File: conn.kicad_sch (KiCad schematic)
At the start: 57 parts, among them J1 JST_1x02, J10 MicroFit_2x04, J11 MLX_1x03, J12 MLX_1x03, J13 JST_1x04, J14 JST_1x04, J15 JST_1x04, J16 JST_1x04, J17 JST_1x02, J5 JST_01x02, J7 JST_B6B-XH, J8 MicroFit_2x04, J9 MicroFit_2x04, SW2 !EMERG STOP!

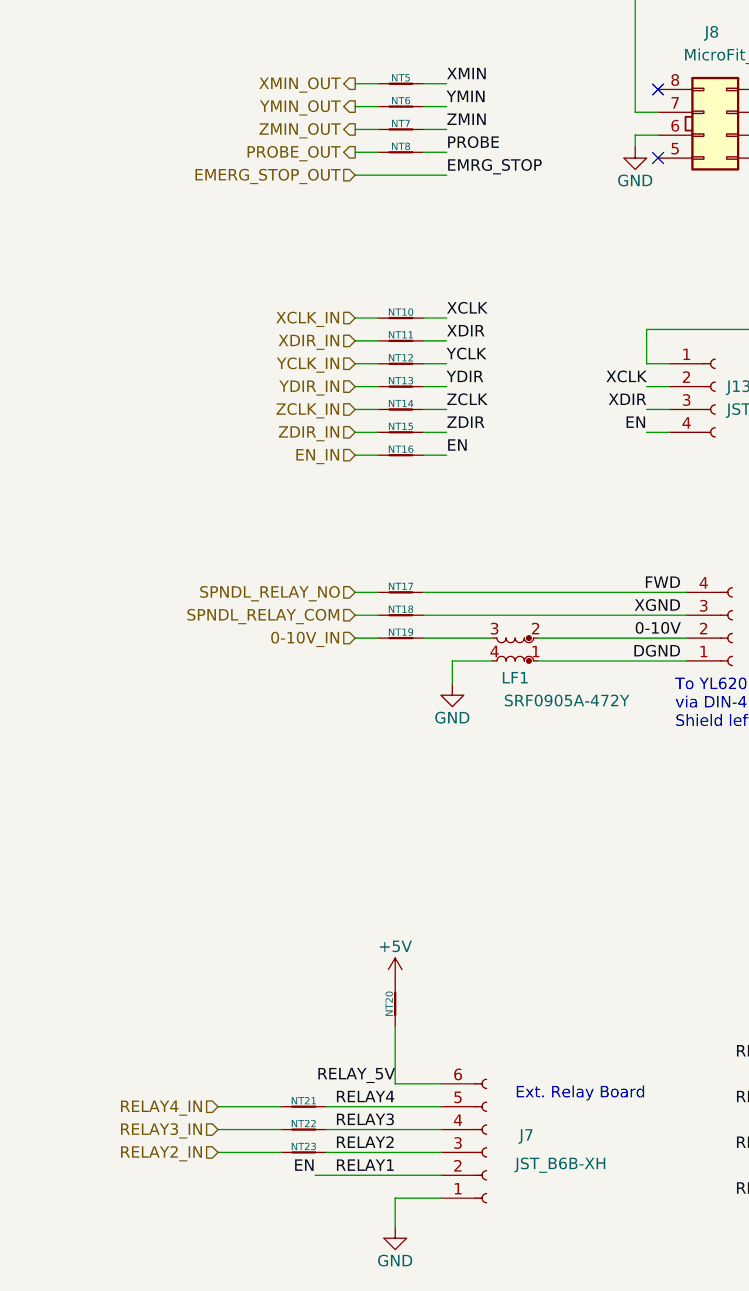
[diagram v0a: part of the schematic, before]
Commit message: Forgot R1 and more NT fun.
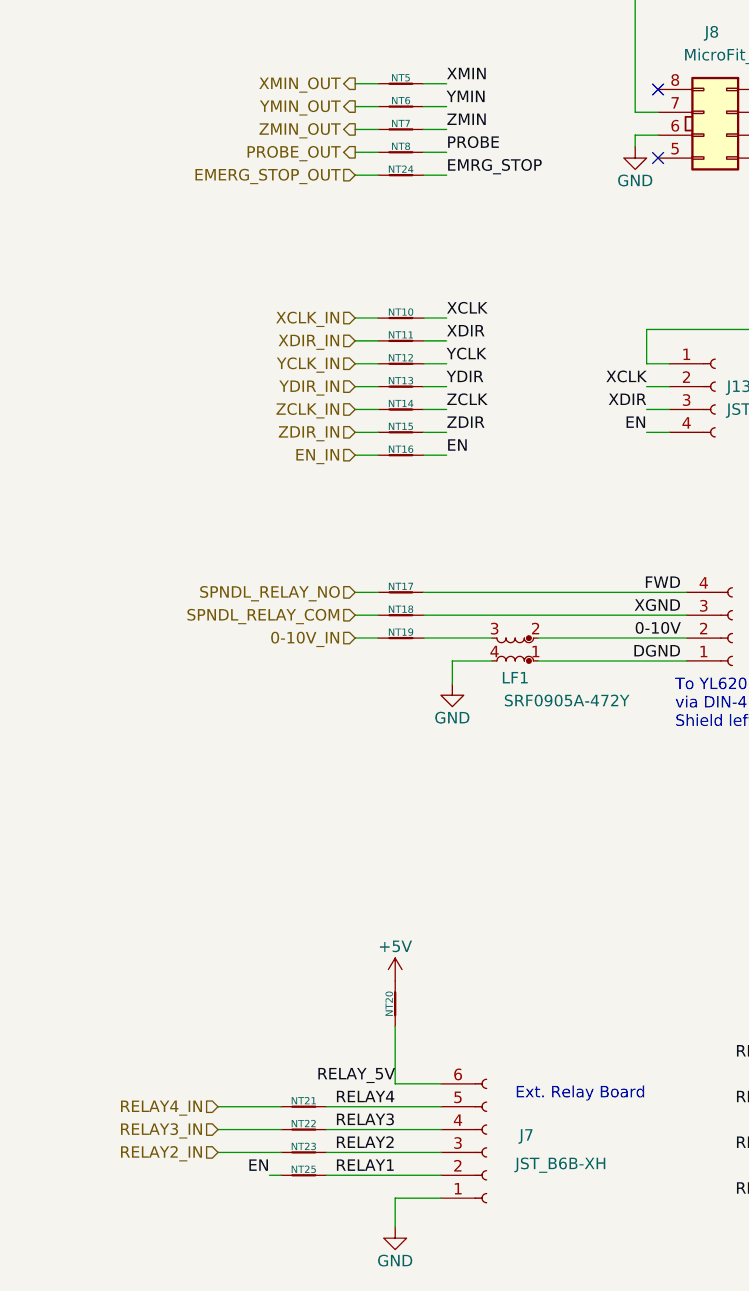
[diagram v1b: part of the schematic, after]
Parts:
- added NT24, NT25: DNI, _footprints:NetTie-2_SMD_Pad0.3mm, symbol Device:NetTie_2
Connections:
- net EMERG_STOP_OUT: now also NT24.1; no longer J1.2 (Pin_2)
- net EN: now also NT25.1; no longer D20.1 (K), J7.2 (Pin_2)
- new net EMRG_STOP: J1.2 (Pin_2), NT24.2
- new net RELAY1: D20.1 (K), J7.2 (Pin_2), NT25.2
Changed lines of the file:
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@@
+    (stroke (width 0) (type default) (color 0 0 0 0))
+  )
+  (wire (pts (xy 53.34 172.72) (xy 66.04 172.72))
     (stroke (width 0) (type default) (color 0 0 0 0))
   )
@@
     (stroke (width 0) (type default) (color 0 0 0 0))
   )
-  (wire (pts (xy 56.515 61.595) (xy 66.675 61.595))
+  (wire (pts (xy 56.515 61.595) (xy 59.055 61.595))
     (stroke (width 0) (type default) (color 0 0 0 0))
   )
@@
     (stroke (width 0) (type default) (color 0 0 0 0))
   )
+  (wire (pts (xy 46.99 172.72) (xy 48.26 172.72))
+    (stroke (width 0) (type default) (color 0 0 0 0))
+  )
   (wire (pts (xy 53.34 170.18) (xy 66.04 170.18))
     (stroke (width 0) (type default) (color 0 0 0 0))
@@
     (stroke (width 0) (type default) (color 0 0 0 0))
   )
+  (wire (pts (xy 64.135 61.595) (xy 66.675 61.595))
+    (stroke (width 0) (type default) (color 0 0 0 0))
+  )
   (wire (pts (xy 197.485 125.73) (xy 204.47 125.73))
     (stroke (width 0) (type default) (color 0 0 0 0))
@@
   )
   (wire (pts (xy 248.92 44.45) (xy 250.19 44.45))
-    (stroke (width 0) (type default) (color 0 0 0 0))
-  )
-  (wire (pts (xy 52.07 172.72) (xy 66.04 172.72))
     (stroke (width 0) (type default) (color 0 0 0 0))
   )
@@
     (effects (font (size 1.27 1.27)) (justify right bottom))
   )
-  (label "EN" (at 52.07 172.72 180)
+  (label "EN" (at 46.99 172.72 180)
     (effects (font (size 1.27 1.27)) (justify right bottom))
   )
@@
     )
     (property "Datasheet" "~" (id 3) (at 146.05 100.33 0)
+      (effects (font (size 1.27 1.27)) hide)
+    )
+    (pin "1")
+    (pin "2")
+  )
+  (symbol (lib_id "Device:NetTie_2") (at 50.8 172.72 0) (unit 1)
+    (in_bom yes) (on_board yes)
+    (property "Reference" "NT25" (id 0) (at 50.8 172.085 0)
+      (effects (font (size 0.8 0.8)))
+    )
+    (property "Value" "DNI" (id 1) (at 50.8 170.18 0)
+      (effects (font (size 1.27 1.27)) hide)
+    )
+    (property "Footprint" "_footprints:NetTie-2_SMD_Pad0.3mm" (id 2) (at 50.8 172.72 0)
+      (effects (font (size 1.27 1.27)) hide)
+    )
+    (property "Datasheet" "~" (id 3) (at 50.8 172.72 0)
       (effects (font (size 1.27 1.27)) hide)
     )
@@
       (effects (font (size 1.27 1.27)) hide)
     )
+    (pin "1")
+    (pin "2")
+  )
+  (symbol (lib_id "Device:NetTie_2") (at 61.595 61.595 0) (unit 1)
+    (in_bom yes) (on_board yes)
+    (property "Reference" "NT24" (id 0) (at 61.595 60.96 0)
+      (effects (font (size 0.8 0.8)))
+    )
+    (property "Value" "DNI" (id 1) (at 61.595 59.055 0)
+      (effects (font (size 1.27 1.27)) hide)
+    )
+    (property "Footprint" "_footprints:NetTie-2_SMD_Pad0.3mm" (id 2) (at 61.595 61.595 0)
+      (effects (font (size 1.27 1.27)) hide)
+    )
+    (property "Datasheet" "~" (id 3) (at 61.595 61.595 0)
+      (effects (font (size 1.27 1.27)) hide)
+    )
